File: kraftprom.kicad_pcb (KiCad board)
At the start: 2 copper layers, 67.5 x 86.2 mm, 21 parts, among them J1 Jumper_3_Bridged12, J2 PROGRAM, U1 PIC16F628A, U2 74HC164, U3 74HC164, U4 74HC164, U5 74LS245, U6 74LS165, U7 FTDI USB ADAPTER

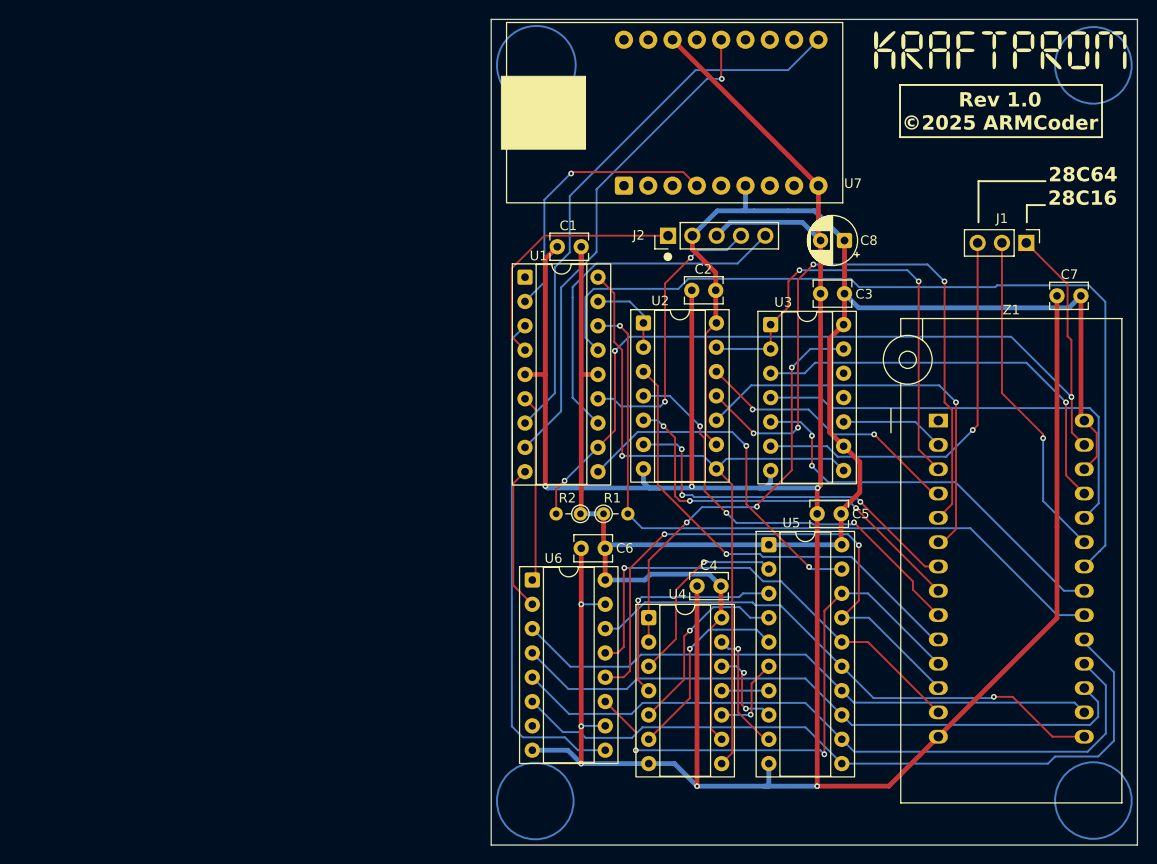
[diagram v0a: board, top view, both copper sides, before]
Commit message: More PCB fixes.
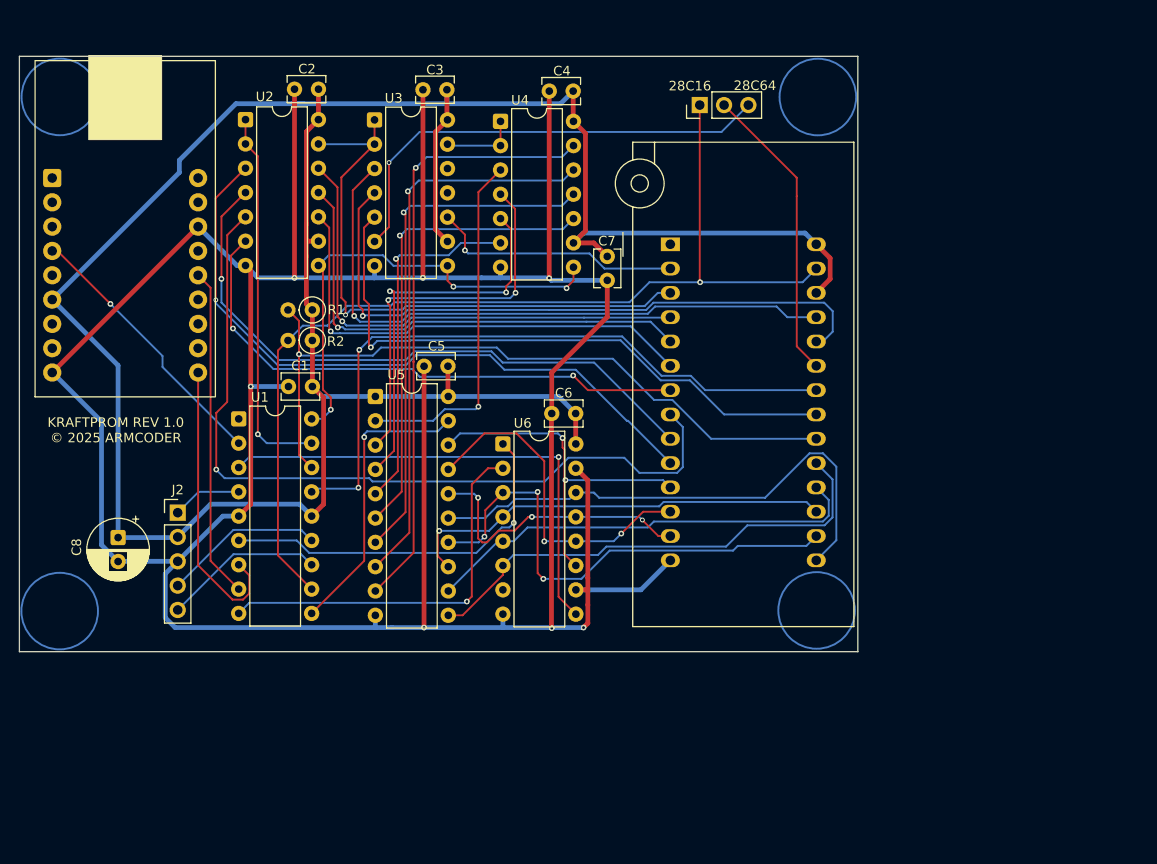
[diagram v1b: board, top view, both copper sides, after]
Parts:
- removed G***: LOGO, Kraft80:kraftprom
- C8: footprint Capacitor_THT:CP_Radial_D5.0mm_P2.50mm -> Capacitor_THT:CP_Radial_D6.3mm_P2.50mm
- R1, R2: footprint Resistor_THT:R_Axial_DIN0204_L3.6mm_D1.6mm_P2.54mm_Vertical -> Resistor_THT:R_Axial_DIN0207_L6.3mm_D2.5mm_P2.54mm_Vertical
- U1: footprint Package_DIP:DIP-18_W7.62mm_Socket -> Package_DIP:DIP-18_W7.62mm
- U2, U3, U4: footprint Package_DIP:DIP-14_W7.62mm_Socket -> Package_DIP:DIP-14_W7.62mm
- U5: footprint Package_DIP:DIP-20_W7.62mm_Socket -> Package_DIP:DIP-20_W7.62mm
- U6: footprint Package_DIP:DIP-16_W7.62mm_Socket -> Package_DIP:DIP-16_W7.62mm
- U7: footprint Kraft80:FTDI-ADAPTER -> KraftPROM:FTDI-ADAPTER
- Z1: footprint Socket:DIP_Socket-28_W11.9mm_W12.7mm_W15.24mm_W17.78mm_W18.5mm_3M_228-1277-00-0602J -> Socket:DIP_Socket-28_W11.9_W12.7_W15.24_W17.78_W18.5_3M_228-1277-00-0602J
- moved C8 82.0 mm to (49.5, 111.1), turned to -90 degrees
- moved J2 58.8 mm to (55.8, 108.5), turned to 0 degrees
- moved U7 55.4 mm to (50.3, 76.1), turned to 90 degrees
- moved U4 54.1 mm to (89.5, 67.7)
- moved C4 54.0 mm to (97.1, 64.5)
- moved C7 49.7 mm to (100.6, 81.8), turned to -90 degrees
- moved U2 46.7 mm to (62.8, 67.5)
- moved C3 46.7 mm to (83.9, 64.3)
- moved U3 46.6 mm to (76.3, 67.5)
- moved C2 46.5 mm to (70.5, 64.3)
- moved U5 43.9 mm to (76.4, 96.4)
- moved C5 43.9 mm to (84.0, 93.2)
- moved R1 37.1 mm to (69.8, 87.3), turned to 180 degrees
- moved J1 37.0 mm to (110.3, 66.0), turned to 90 degrees
- moved Z1 33.5 mm to (107.2, 80.5)
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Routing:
- net +5V: track 220.9 -> 271.9 mm
- net Net-(U4-Q7): track 13.0 -> 63.4 mm
- net Net-(U4-Q6): track 9.28 -> 59.0 mm, vias 2 -> 1
- net Net-(U4-Q5): track 4.93 -> 54.4 mm, vias 0 -> 1
- net Net-(U2-Q2): track 41.8 -> 84.9 mm, vias 3 -> 1
- net Net-(U4-Q4): track 9.26 -> 49.6 mm
- net Net-(U3-Q7): track 44.4 -> 8.14 mm, vias 3 -> 0
- net /PGDAT: track 8.69 -> 39.4 mm, vias 0 -> 1
- net Net-(U1-RB1/RX/DT): track 58.4 -> 30.7 mm
- net /PGCLK: track 76.3 -> 49.5 mm, vias 1 -> 3
- net Net-(U5-B6): track 73.1 -> 46.5 mm
- net Net-(U5-B7): track 77.2 -> 51.5 mm
- net /VERCLK: track 15.2 -> 40.7 mm, vias 0 -> 1
- net Net-(U5-B1): track 61.0 -> 35.6 mm
- net Net-(U2-Q6): track 28.6 -> 51.8 mm, vias 2 -> 1
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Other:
- board size 67.5 x 86.2 mm -> 87.6 x 62.2 mm
- board text added: "KRAFTPROM REV 1.0 © 2025 ARMCODER"
- board text removed: "Rev 1.0 ©2025 ARMCoder"
